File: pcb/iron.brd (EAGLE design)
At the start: 8 x 48 mm, 22 parts, among them IC1 AT24CS04-SOT23, IC2 TS507CLT, IC3 AD7995, IC4 ESDA6V1SC5, X1 LUMBERG_KLB_4

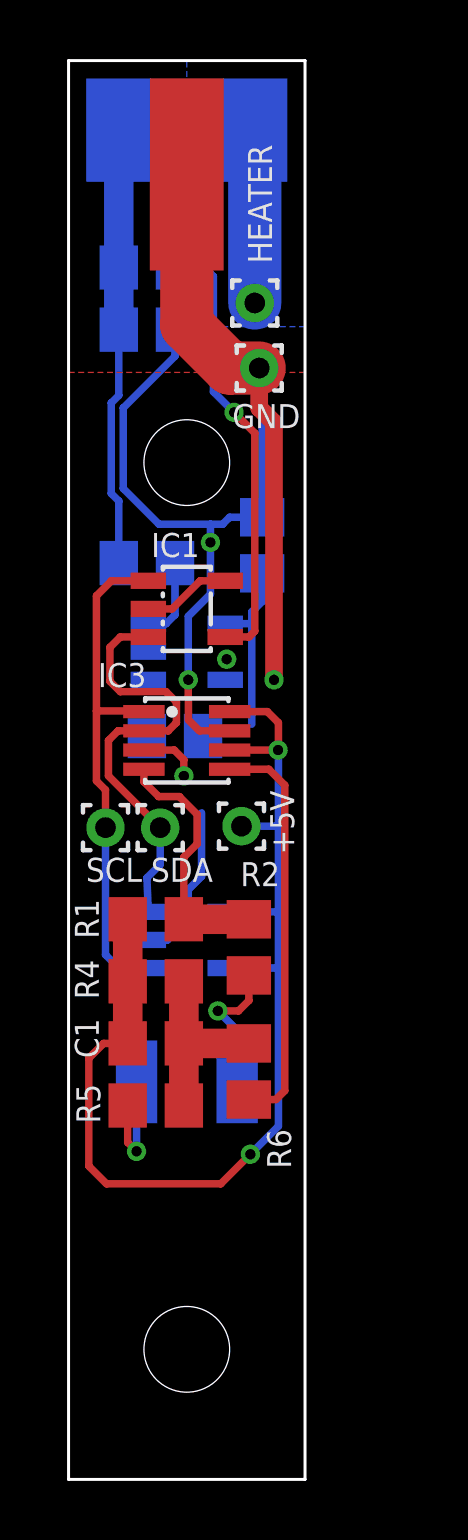
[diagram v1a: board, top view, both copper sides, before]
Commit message: iron drills deleted
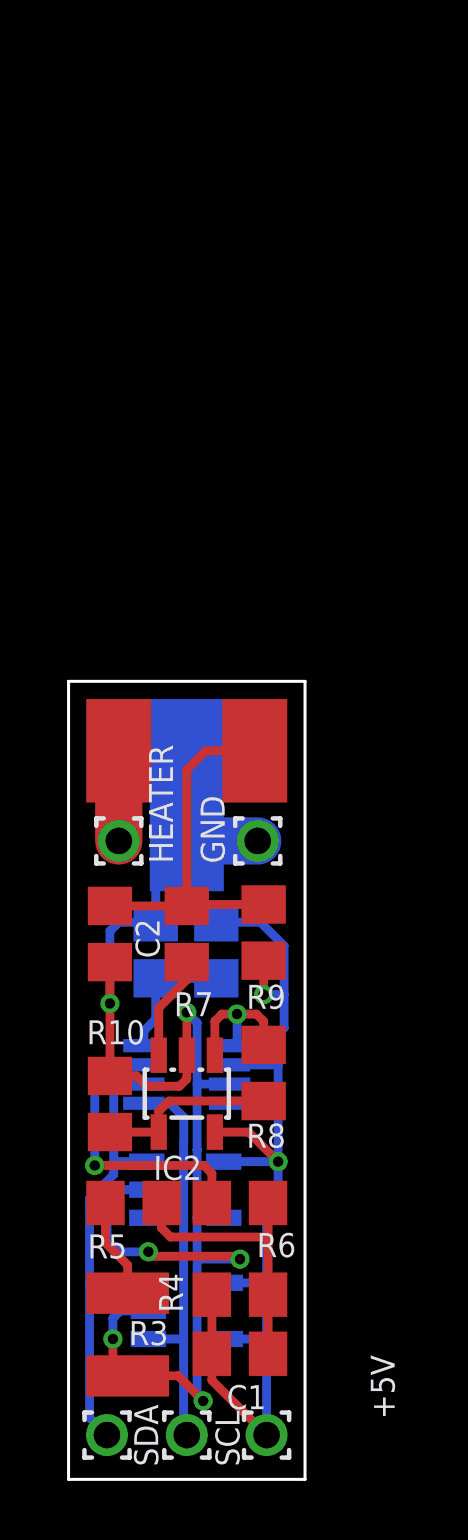
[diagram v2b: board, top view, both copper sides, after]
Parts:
- moved R9 22.8 mm to (6.60, 18.5), flipped to the top, turned to 270 degrees
- moved X1 21.0 mm to (4.00, 26.4), flipped to the bottom
- moved SCL 20.7 mm to (4.00, 1.50)
- moved SDA 20.6 mm to (1.30, 1.50)
- moved +5V 20.6 mm to (6.70, 1.50)
- moved C2 20.5 mm to (1.40, 18.4), flipped to the top, turned to 270 degrees
- moved IC1 19.7 mm to (3.95, 9.80), flipped to the bottom, turned to 90 degrees
- moved R10 19.6 mm to (1.40, 12.7), flipped to the top
- moved HEATER 18.8 mm to (1.70, 21.6)
- moved GND 16.0 mm to (6.40, 21.6)
- moved IC2 14.9 mm to (4.00, 13.1), flipped to the top, turned to 180 degrees
- moved R7 12.6 mm to (4.00, 18.4), flipped to the top, turned to 90 degrees
- moved IC4 12.6 mm to (4.00, 5.70)
- moved R8 11.8 mm to (6.60, 13.8), flipped to the top, turned to 90 degrees
- moved IC3 11.3 mm to (4.00, 13.7), flipped to the bottom, turned to 90 degrees
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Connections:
- net AD_MOTION: now also IC3.3; no longer IC3.5
- net AD_TC: now also IC3.5; no longer IC3.3
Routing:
- net +5V: track 53.9 -> 37.3 mm, vias 4 -> 2
- net GND: track 57.0 -> 51.4 mm, vias 4 -> 6
- net AD_COMP: track 8.62 -> 4.49 mm
- net AD_MOTION: track 13.8 -> 9.77 mm, vias 0 -> 1
- net MOTION_FIL: track 6.40 -> 9.67 mm
- net AD_TC: track 2.03 -> 5.12 mm
- net HEATER: track 5.85 -> 3.05 mm
- net SCL: track 17.5 -> 14.8 mm
- net THERMO_UNFIL: track 14.9 -> 12.4 mm
- net SDA: track 15.1 -> 16.5 mm
- net THERMO_FIL: track 2.77 -> 3.54 mm
- net MOTION_DIV: track 4.02 -> 3.36 mm, vias 1 -> 0
- removed copper zone on layer 1, net +5V
- removed copper zone on layer 1, net GND
- removed copper zone on layer 16, net GND
- removed copper zone on layer 16, net HEATER
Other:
- board size 8 x 48 mm -> 8 x 27 mm

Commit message: parts reworked
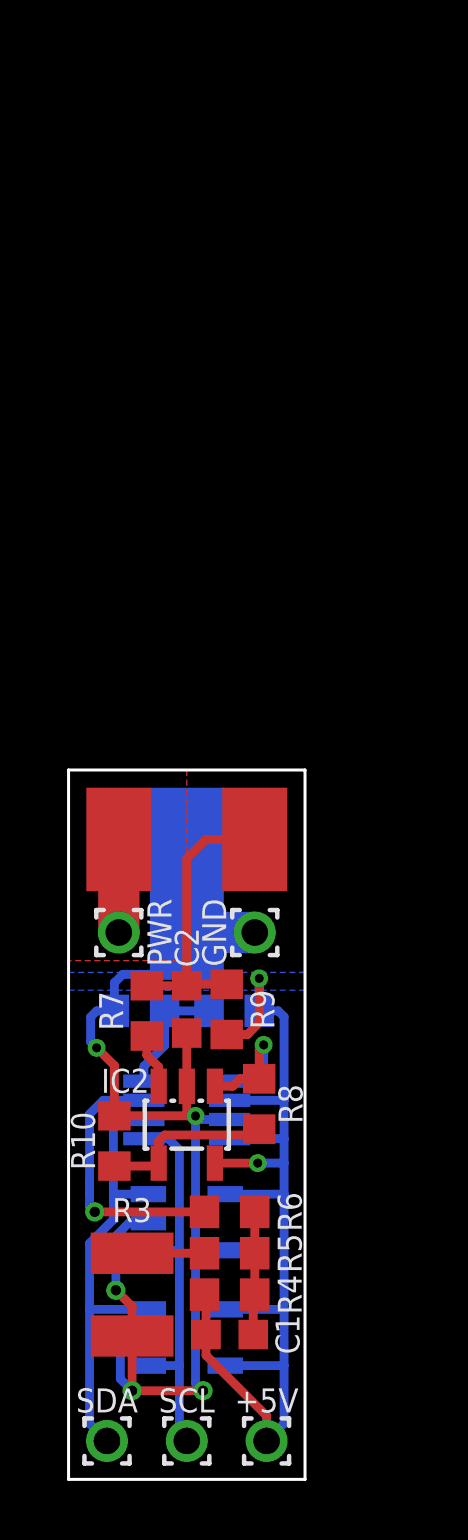
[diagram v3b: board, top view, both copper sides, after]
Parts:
- removed HEATER: (no value), solderpi:1,6/0,8
- added PWR: (no value), solderpi:1,6/0,8
- C1, C2: device rcl:C0805 -> common:C0603
- R1, R4, R5, R6, R7, R8, R9: device rcl:R0805 -> common:R0603
- R10: value 2k 0,1% -> 2k 0.1%; device rcl:R0805 -> common:R0603
- R2: value 68k @25°C, 1%, ß=4100 K -> 68k @25°C, 1%, ß=3985 K; device solderpi:R0805 -> common:R0603
- moved R5 3.67 mm to (5.45, 7.65)
- moved C2 3.64 mm to (4.00, 15.9)
- moved GND 3.10 mm to (6.30, 18.5)
- moved X1 3.00 mm to (4.00, 23.4)
- moved R7 2.93 mm to (2.65, 15.8)
- moved R9 2.88 mm to (5.35, 15.9)
- moved R1 2.14 mm to (5.60, 15.8), turned to 180 degrees
- moved R2 2.12 mm to (2.40, 15.8), turned to 180 degrees
- moved R3 1.36 mm to (2.15, 6.25)
- moved R10 1.26 mm to (1.55, 11.4)
- moved IC3 1.20 mm to (4.00, 12.5)
- moved IC1 1.10 mm to (4.00, 8.70)
- moved R8 1.06 mm to (6.45, 12.7)
- moved IC2 1.05 mm to (4.00, 12.0)
- moved IC4 0.90 mm to (4.00, 4.80)
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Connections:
- net HEATER: now also PWR.1; no longer HEATER.1
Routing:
- net GND: track 51.4 -> 42.6 mm, vias 6 -> 5
- net MOTION_FIL: track 9.67 -> 4.20 mm
- net THERMO_UNFIL: track 12.4 -> 9.59 mm
- net THERMO_FIL: track 3.54 -> 1.87 mm
- net SCL: track 14.8 -> 13.4 mm
- net SDA: track 16.5 -> 15.5 mm
- net MOTION_DIV: track 3.36 -> 2.45 mm
- net AD_MOTION: track 9.77 -> 9.13 mm
- added copper zone on layer 1, net GND
- added copper zone on layer 16, net GND
- added copper zone on layer 1, net HEATER
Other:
- board size 8 x 27 mm -> 8 x 24 mm
